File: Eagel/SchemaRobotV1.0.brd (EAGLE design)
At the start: 137 x 79 mm, 25 parts, among them J1 Connector US1, J2 Connector US 2, J3 Connector US 2, J4 Connector H-Brug, J5 Connector IR voeding, J6 Connector IR signalen, J7 Connector batterij 12v, J8 Connector LCD, J9 Connector HC-05

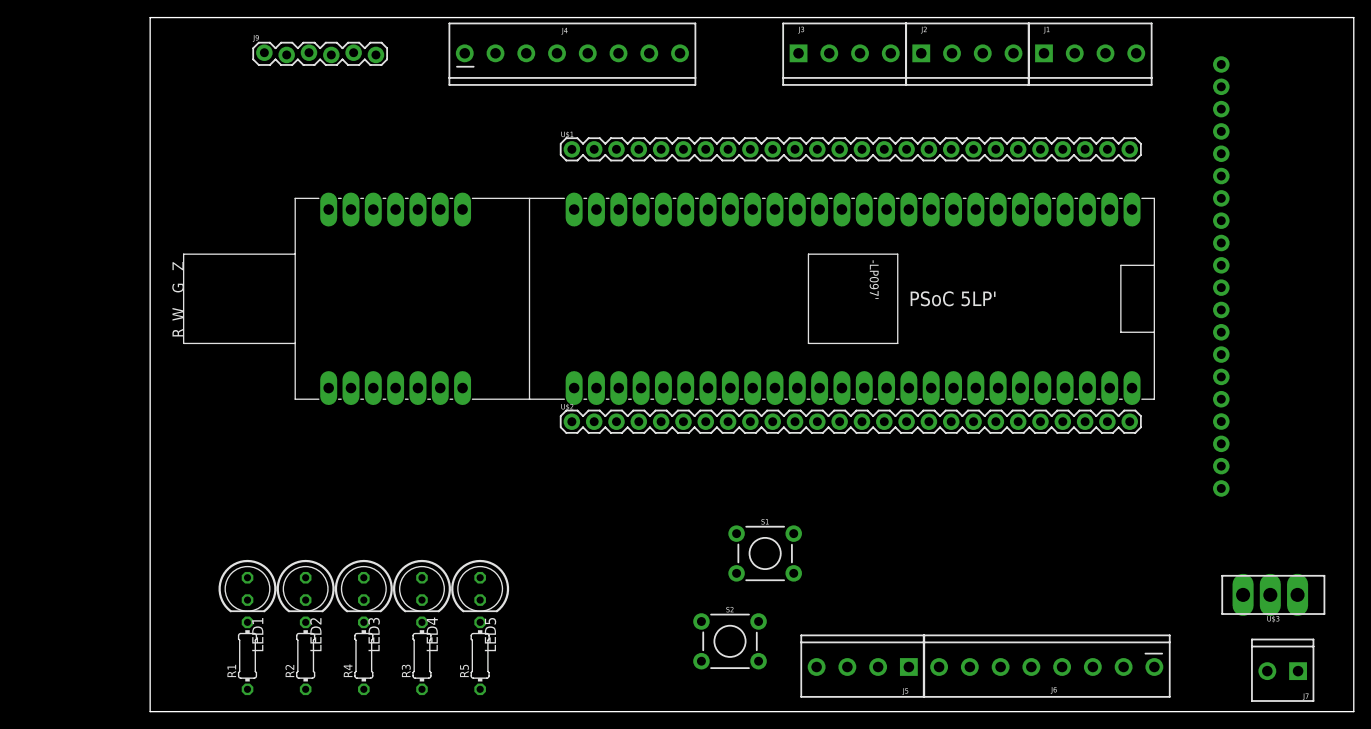
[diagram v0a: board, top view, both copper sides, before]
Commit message: eagle
pcb bijna af
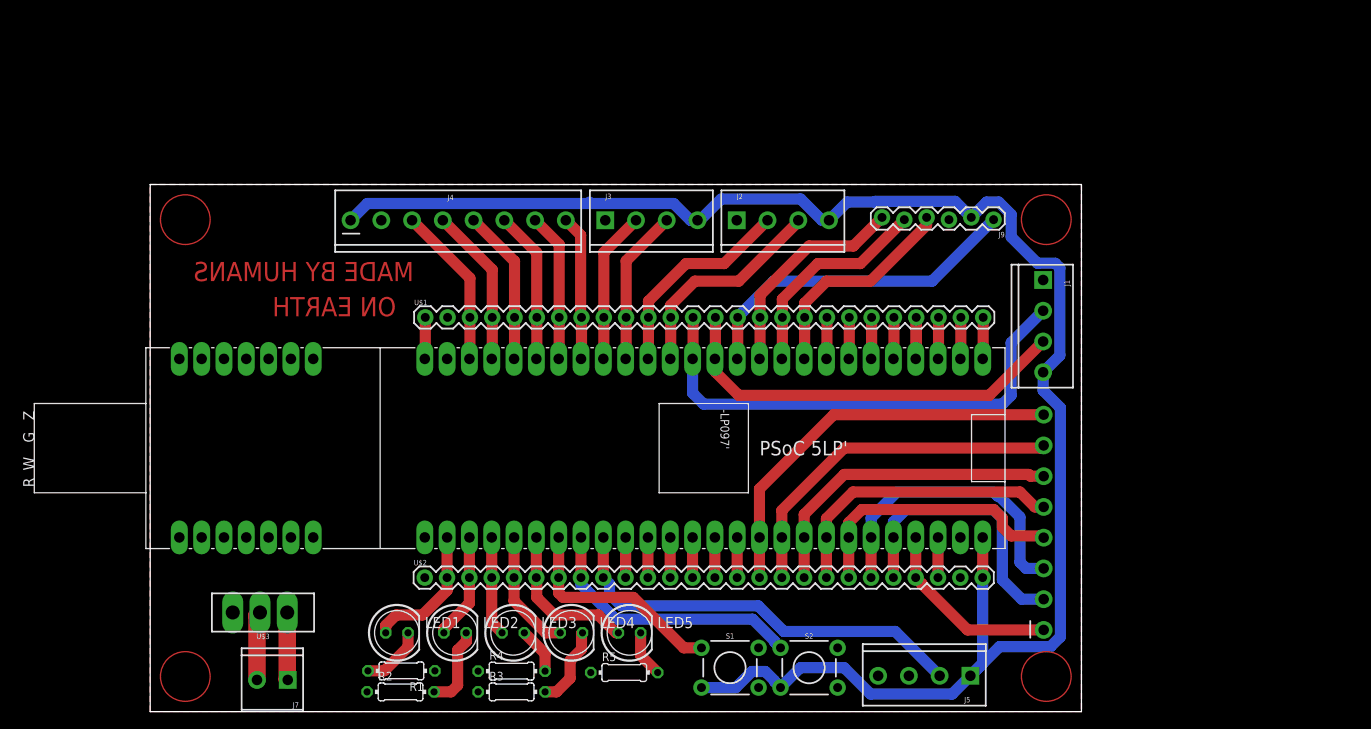
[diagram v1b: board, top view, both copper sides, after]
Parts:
- removed J8: Connector LCD, SparkFun-Connectors:1X20
- moved U$3 115.0 mm to (7.00, 9.00)
- moved J7 115.0 mm to (15.7, 3.61)
- moved J9 85.1 mm to (96.0, 56.0), turned to 180 degrees
- moved J3 29.1 mm to (51.8, 55.9)
- moved J2 28.3 mm to (66.8, 55.9)
- moved J1 25.8 mm to (101.6, 49.1), turned to 270 degrees
- moved U$1 25.4 mm to (31.3, 44.9)
- moved U$2 24.4 mm to (31.3, 15.3)
- moved DEVICE1 24.0 mm to (47.8, 30.0)
- moved J4 23.0 mm to (22.8, 55.9)
- moved LED2 17.7 mm to (34.7, 8.97), turned to 0 degrees
- moved LED1 17.7 mm to (28.1, 8.97), turned to 0 degrees
- moved LED3 17.7 mm to (41.3, 8.97), turned to 0 degrees
- moved LED5 17.7 mm to (54.6, 8.97), turned to 0 degrees
- moved LED4 17.7 mm to (47.9, 8.97), turned to 0 degrees
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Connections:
- net GND: no longer J8.1, J8.3
- net P2.0: no longer J8.11
- net P2.1: no longer J8.12
- net P2.2: no longer J8.13
- net P2.3: no longer J8.14
- net P2.4: no longer J8.6
- net P2.5: no longer J8.4
- net P2.6: no longer J8.5
- net VCC: no longer J8.2
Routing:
- net VCC: track 0.00 -> 198.8 mm
- net P12.2: track 0.00 -> 57.0 mm
- net P3.7: track 0.00 -> 48.2 mm
- net P12.3: track 0.00 -> 47.2 mm
- net P0.0: track 0.00 -> 46.0 mm
- net P0.1: track 0.00 -> 40.5 mm
- net P12.4: track 0.00 -> 38.5 mm
- net P0.2: track 0.00 -> 36.4 mm
- net P0.5: track 0.00 -> 34.3 mm
- net P0.3: track 0.00 -> 33.4 mm
- net P0.6: track 0.00 -> 32.4 mm
- net P3.6: track 0.00 -> 31.1 mm
- net P0.4: track 0.00 -> 31.0 mm
- net P3.5: track 0.00 -> 25.2 mm
- net P12.5: track 0.00 -> 24.8 mm
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- added copper zone on layer 1, net GND
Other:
- board size 137 x 79 mm -> 106 x 60 mm
- board text added: "MADE BY HUMANS"
- board text added: "ON EARTH"
